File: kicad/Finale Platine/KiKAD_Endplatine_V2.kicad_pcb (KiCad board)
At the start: 2 copper layers, 100 x 80 mm, 70 parts, among them J1 Conn_02x08_Odd_Even, J4 Conn_01x03_Pin, Q1 Q_NPN_ECB, Q2 Q_NPN_ECB, Q3/+1/+1 Q_NPN_ECB, U1 NE555P, U2 TL074

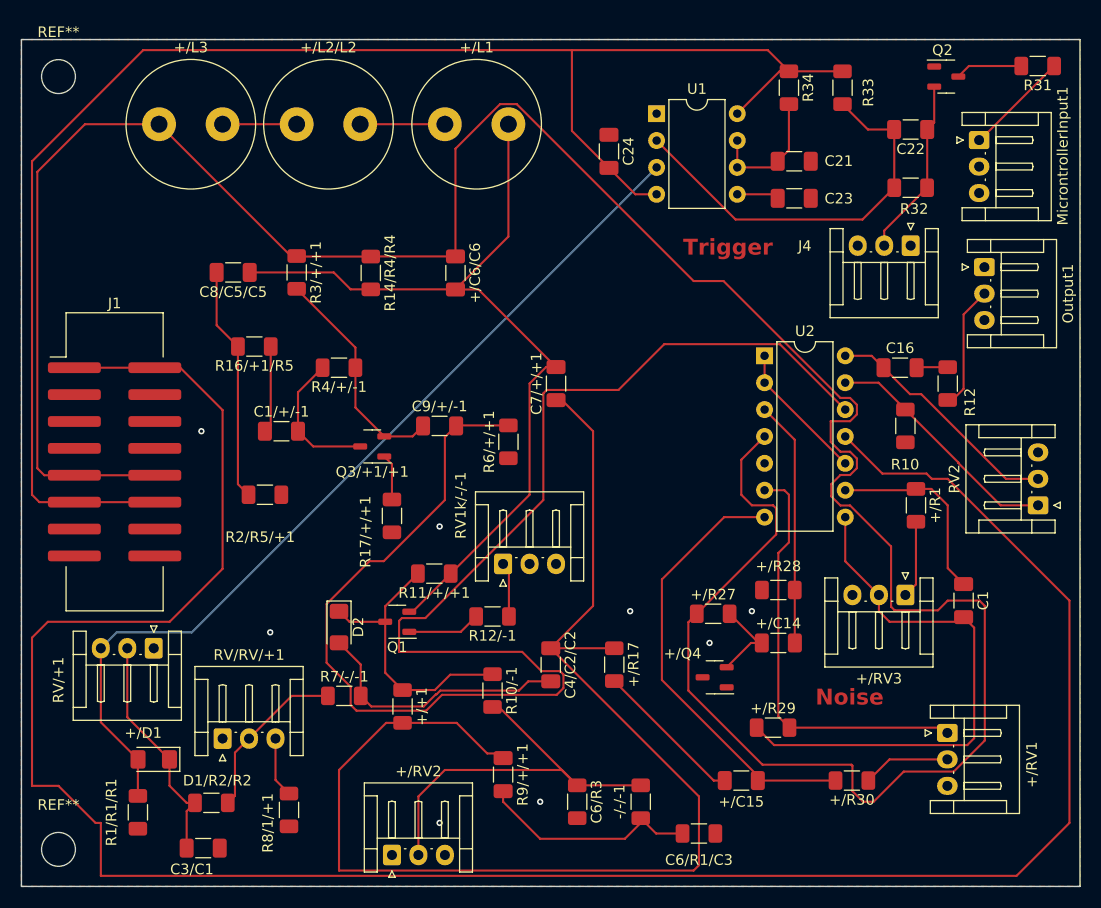
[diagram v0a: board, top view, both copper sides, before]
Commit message: alles mögliche
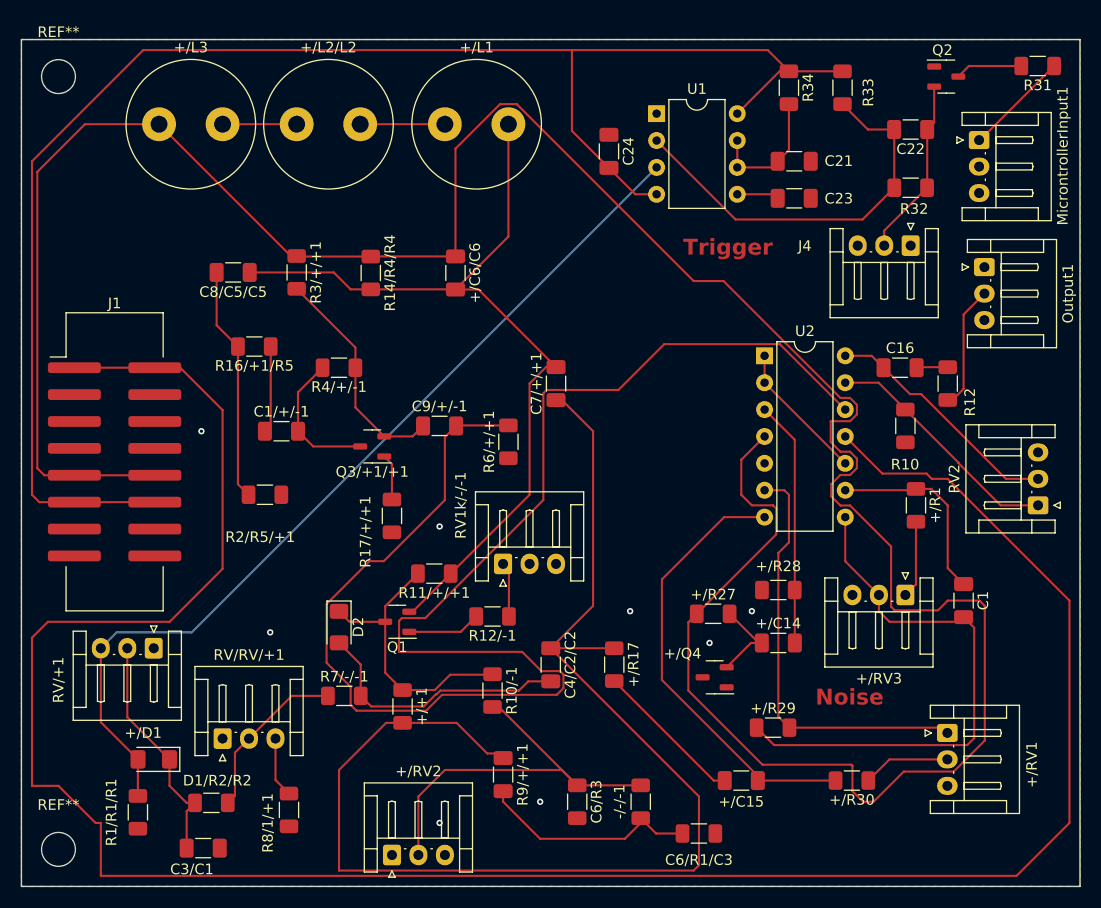
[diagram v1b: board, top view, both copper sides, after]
